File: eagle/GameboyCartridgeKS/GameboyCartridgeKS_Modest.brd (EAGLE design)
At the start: 49.3 x 48 mm, 27 parts, among them IC2 MEGA64-A, Y1 16MHz max

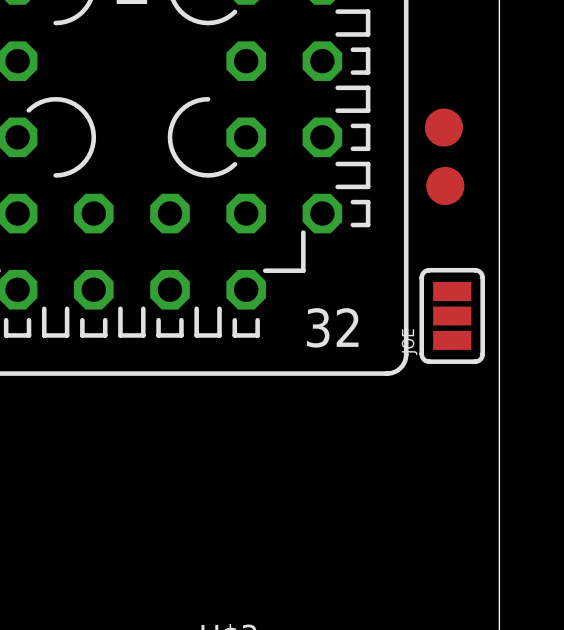
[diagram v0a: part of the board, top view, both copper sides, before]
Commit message: Minor edit
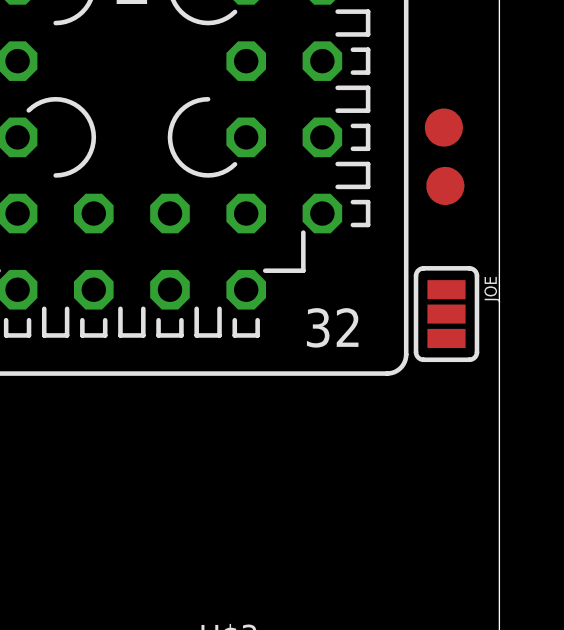
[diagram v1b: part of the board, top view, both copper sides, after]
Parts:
- moved JOE 0.20 mm to (48.4, 26.7), turned to 270 degrees
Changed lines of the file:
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@@
 <element name="SCL3" library="SparkFun-Passives" package="PAD.03X.05" value="" x="6.7945" y="8.763"/>
 <element name="SCL4" library="SparkFun-Passives" package="PAD.03X.05" value="" x="8.1915" y="10.4775"/>
-<element name="JOE" library="SparkFun-Passives" package="PAD-JUMPER-3-NO_YES_SILK" value="" x="48.5775" y="26.6065" rot="R90"/>
+<element name="JOE" library="SparkFun-Passives" package="PAD-JUMPER-3-NO_YES_SILK" value="" x="48.387" y="26.67" rot="R270"/>
 </elements>
 <signals>
@@
 <wire x1="9.43" y1="26.49" x2="6.23" y2="42.09" width="0" layer="19" extent="1-1"/>
 <wire x1="18.78" y1="24.67" x2="9.43" y2="26.49" width="0" layer="19" extent="1-1"/>
-<wire x1="11.43" y1="12.97" x2="18.78" y2="24.67" width="0" layer="19" extent="1-1"/>
-<wire x1="6.35" y1="12.97" x2="11.43" y2="12.97" width="0" layer="19" extent="1-1"/>
 <wire x1="26.9" y1="21.59" x2="18.78" y2="24.67" width="0" layer="19" extent="1-1"/>
 <wire x1="36.63" y1="27.48" x2="26.9" y2="21.59" width="0" layer="19" extent="1-1"/>
+<wire x1="11.43" y1="12.97" x2="9.43" y2="26.49" width="0" layer="19" extent="1-1"/>
+<wire x1="6.35" y1="12.97" x2="11.43" y2="12.97" width="0" layer="19" extent="1-1"/>
 <wire x1="48.95" y1="4" x2="36.63" y2="27.48" width="0" layer="19" extent="1-1"/>
 </signal>
@@
 <contactref element="D1" pad="A"/>
 <contactref element="JD1" pad="1"/>
-<wire x1="2.2225" y1="18.727" x2="2.2225" y2="16.637" width="0" layer="19" extent="1-1"/>
+<wire x1="2.2225" y1="16.637" x2="2.2225" y2="18.727" width="0" layer="19" extent="1-1"/>
 <wire x1="2.05" y1="4" x2="2.2225" y2="16.637" width="0" layer="19" extent="1-1"/>
 </signal>
@@
 <contactref element="IC2" pad="30"/>
 <contactref element="SCL4" pad="P$1"/>
-<wire x1="8.25" y1="4" x2="15.83" y2="26.49" width="0" layer="19" extent="1-1"/>
-<wire x1="8.1915" y1="10.4775" x2="8.25" y2="4" width="0" layer="19" extent="1-1"/>
+<wire x1="8.1915" y1="10.4775" x2="15.83" y2="26.49" width="0" layer="19" extent="1-1"/>
+<wire x1="8.25" y1="4" x2="8.1915" y2="10.4775" width="0" layer="19" extent="1-1"/>
 </signal>
 <signal name="!GB_WR">
@@
 <contactref element="IC2" pad="28"/>
 <contactref element="SCL2" pad="P$1"/>
-<wire x1="5.25" y1="4" x2="14.23" y2="26.49" width="0" layer="19" extent="1-1"/>
-<wire x1="5.334" y1="10.3505" x2="5.25" y2="4" width="0" layer="19" extent="1-1"/>
+<wire x1="5.334" y1="10.3505" x2="14.23" y2="26.49" width="0" layer="19" extent="1-1"/>
+<wire x1="5.25" y1="4" x2="5.334" y2="10.3505" width="0" layer="19" extent="1-1"/>
 </signal>
 <signal name="22">
@@
 <contactref element="SCL3" pad="P$1"/>
 <contactref element="JOE" pad="3"/>
-<wire x1="6.75" y1="4" x2="15.03" y2="26.49" width="0" layer="19" extent="1-1"/>
-<wire x1="6.7945" y1="8.763" x2="6.75" y2="4" width="0" layer="19" extent="1-1"/>
-<wire x1="48.5775" y1="27.4193" x2="6.7945" y2="8.763" width="0" layer="19" extent="1-1"/>
+<wire x1="15.03" y1="26.49" x2="48.387" y2="25.8572" width="0" layer="19" extent="1-1"/>
+<wire x1="6.7945" y1="8.763" x2="15.03" y2="26.49" width="0" layer="19" extent="1-1"/>
+<wire x1="6.75" y1="4" x2="6.7945" y2="8.763" width="0" layer="19" extent="1-1"/>
 </signal>
 <signal name="!WE">
@@
 <contactref element="IC2" pad="27"/>
 <contactref element="SCL1" pad="P$1"/>
-<wire x1="3.75" y1="4" x2="13.43" y2="26.49" width="0" layer="19" extent="1-1"/>
-<wire x1="3.683" y1="8.9535" x2="3.75" y2="4" width="0" layer="19" extent="1-1"/>
+<wire x1="3.683" y1="8.9535" x2="13.43" y2="26.49" width="0" layer="19" extent="1-1"/>
+<wire x1="3.75" y1="4" x2="3.683" y2="8.9535" width="0" layer="19" extent="1-1"/>
 </signal>
 <signal name="N$1">
 <contactref element="IC2" pad="26"/>
 <contactref element="SDA" pad="P$1"/>
-<wire x1="16.51" y1="22.86" x2="12.63" y2="26.49" width="0" layer="19" extent="1-1"/>
+<wire x1="12.63" y1="26.49" x2="16.51" y2="22.86" width="0" layer="19" extent="1-1"/>
 </signal>
 <signal name="N$5">
@@
 <contactref element="TP2" pad="P$1"/>
 <contactref element="JOE" pad="2"/>
+<wire x1="48.387" y1="26.67" x2="48.301" y2="32.886" width="0" layer="19" extent="1-1"/>
 <wire x1="41.71" y1="32.56" x2="48.301" y2="32.886" width="0" layer="19" extent="1-1"/>
-<wire x1="48.5775" y1="26.6065" x2="41.71" y2="32.56" width="0" layer="19" extent="1-1"/>
 </signal>
 <signal name="N$7">
 <contactref element="JOE" pad="1"/>
 <contactref element="IC2" pad="14"/>
-<wire x1="48.5775" y1="25.7937" x2="3.63" y2="29.89" width="0" layer="19" extent="1-1"/>
+<wire x1="3.63" y1="29.89" x2="48.387" y2="27.4828" width="0" layer="19" extent="1-1"/>
 </signal>
 </signals>
